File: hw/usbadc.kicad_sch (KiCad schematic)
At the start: 3 parts, among them J4 JTAG

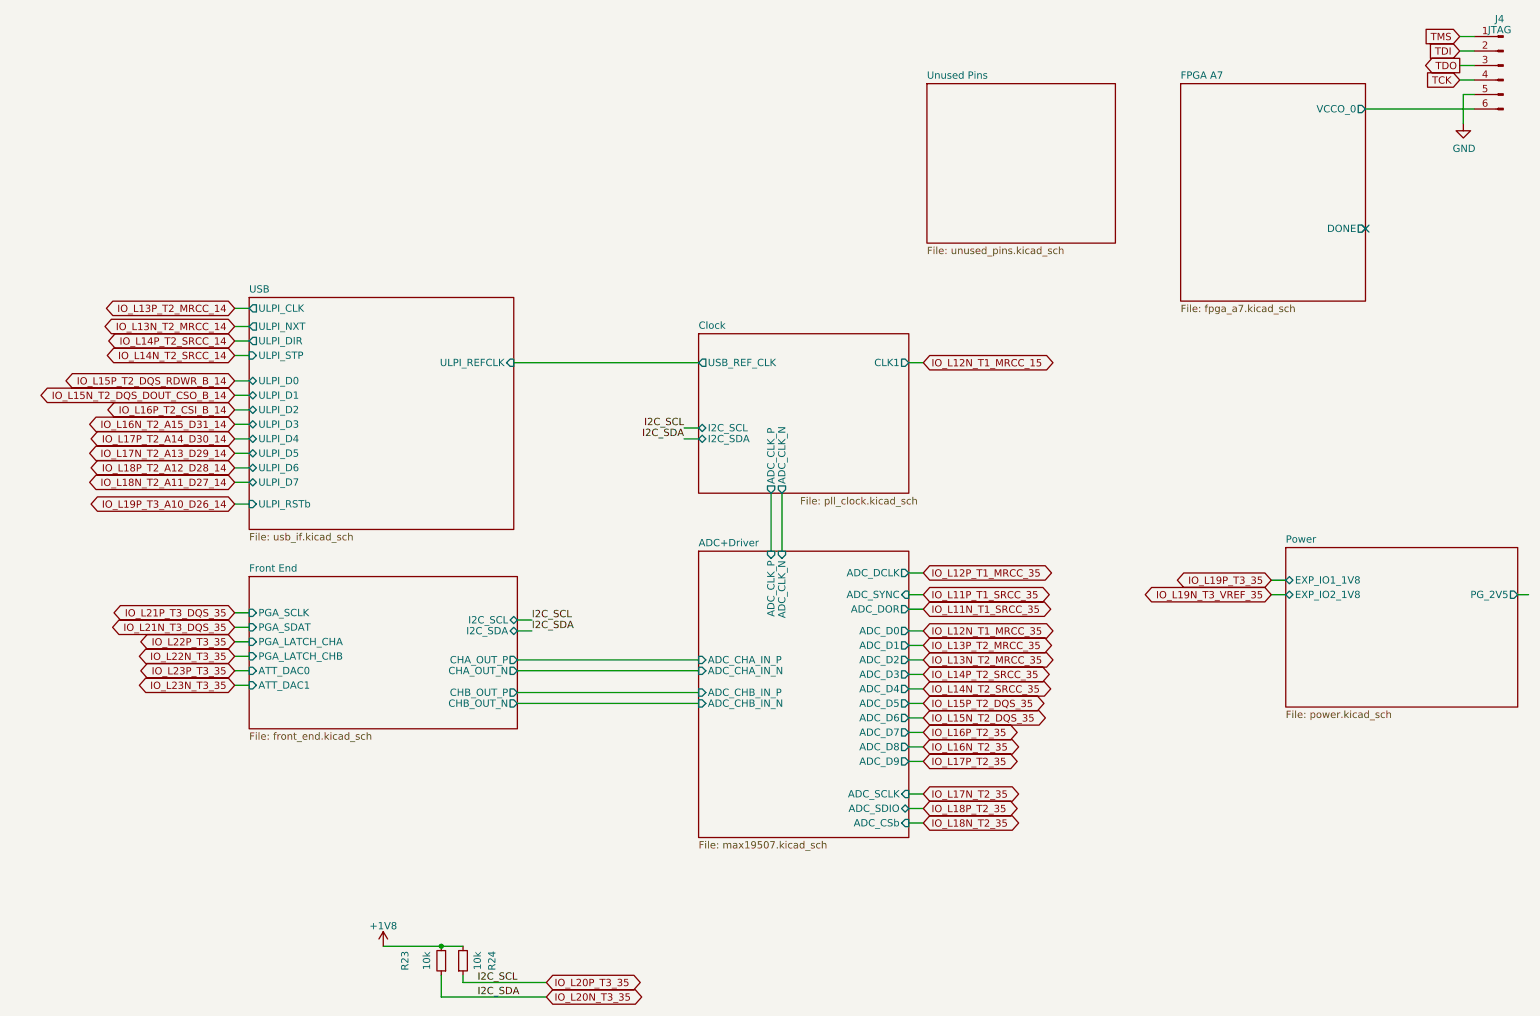
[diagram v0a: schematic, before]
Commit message: WIP (layout)
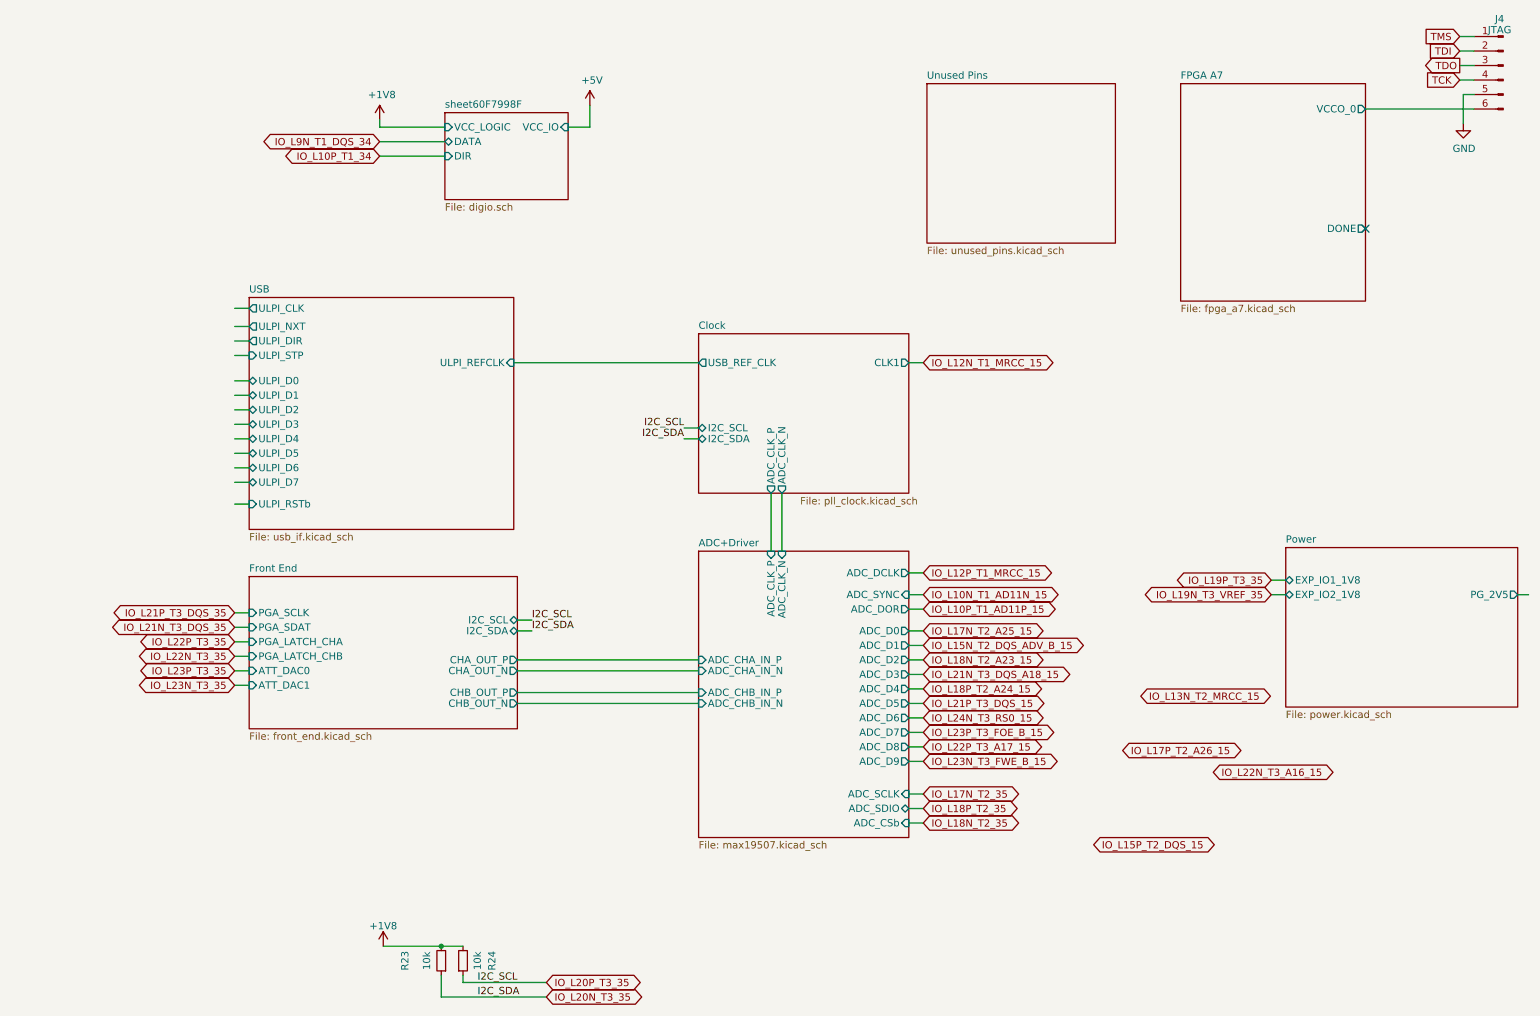
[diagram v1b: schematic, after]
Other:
- added sheet sheet60F7998F (digio.sch)
